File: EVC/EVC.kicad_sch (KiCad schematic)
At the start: 33 parts, among them CN1 HC-ZH1.5-6AW, CN2 HC-ZH1.5-6AW, CN3 HC-ZH1.5-6AW, CN4 HC-ZH1.5-6AW, J1 USB4105-GF-A, J2 screen, P1 WJ500V-5.08-2P-14-00A, Q1 AMS1117-3.3V_C5120796, U1 CH592X, U4 DRV8835DSSR, U5 DRV8835DSSR, X1 Q13FC1350000400, Y1 XRCGB32M000F2P01R0

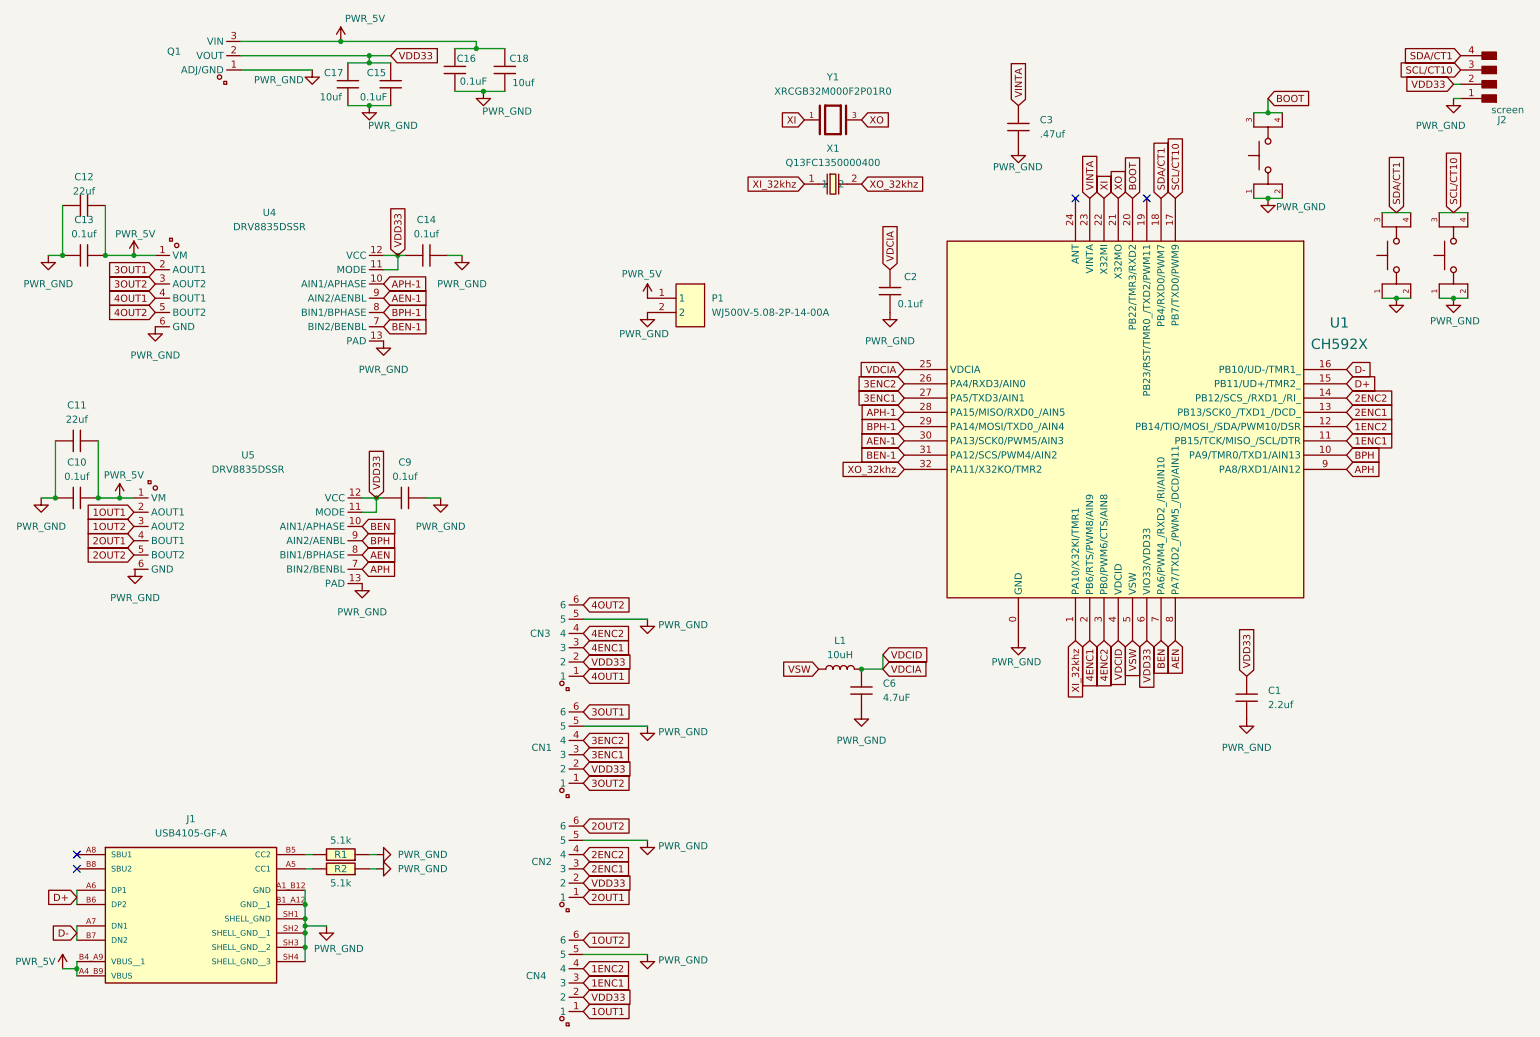
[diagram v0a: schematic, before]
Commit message: fixed some stuff reorder should be aokay
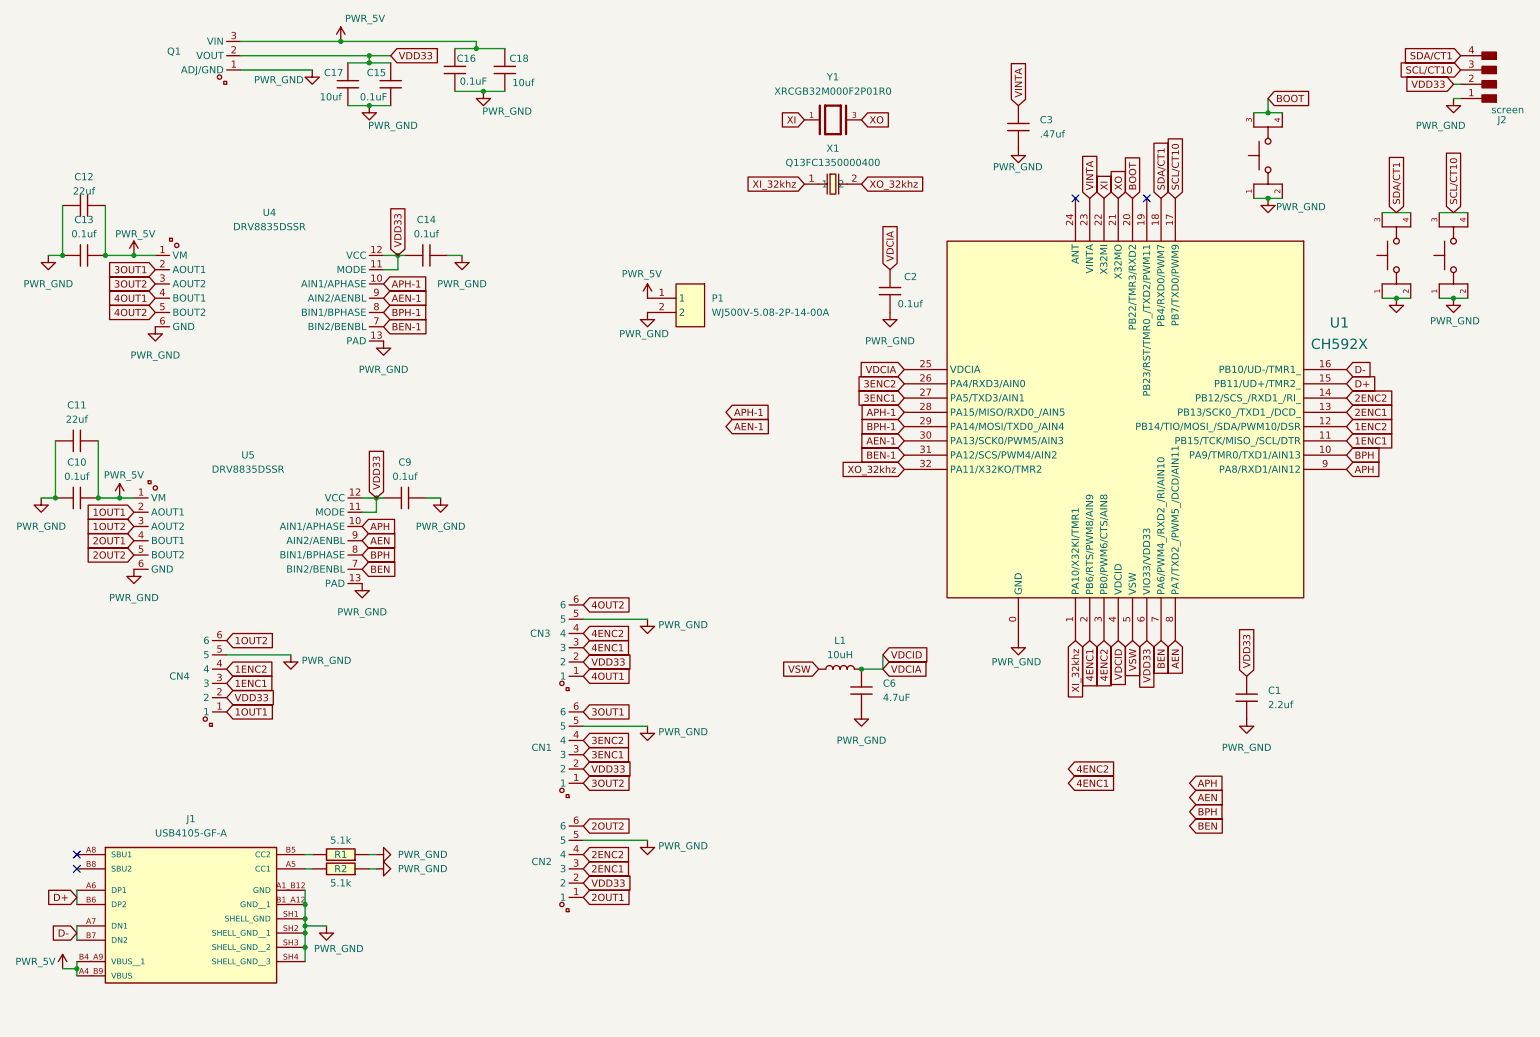
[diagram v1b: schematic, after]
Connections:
- net AEN: now also U5.9 (AIN2/AENBL); no longer U5.8 (BIN1/BPHASE)
- net APH: now also U5.10 (AIN1/APHASE); no longer U5.7 (BIN2/BENBL)
- net BEN: now also U5.7 (BIN2/BENBL); no longer U5.10 (AIN1/APHASE)
- net BPH: now also U5.8 (BIN1/BPHASE); no longer U5.9 (AIN2/AENBL)
- net PWR_GND: now also U5.6 (GND)
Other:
- moved on the sheet: CN4
